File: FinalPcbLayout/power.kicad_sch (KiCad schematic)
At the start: 33 parts, among them Q1 NMOS, U4 AMS1117-3.3

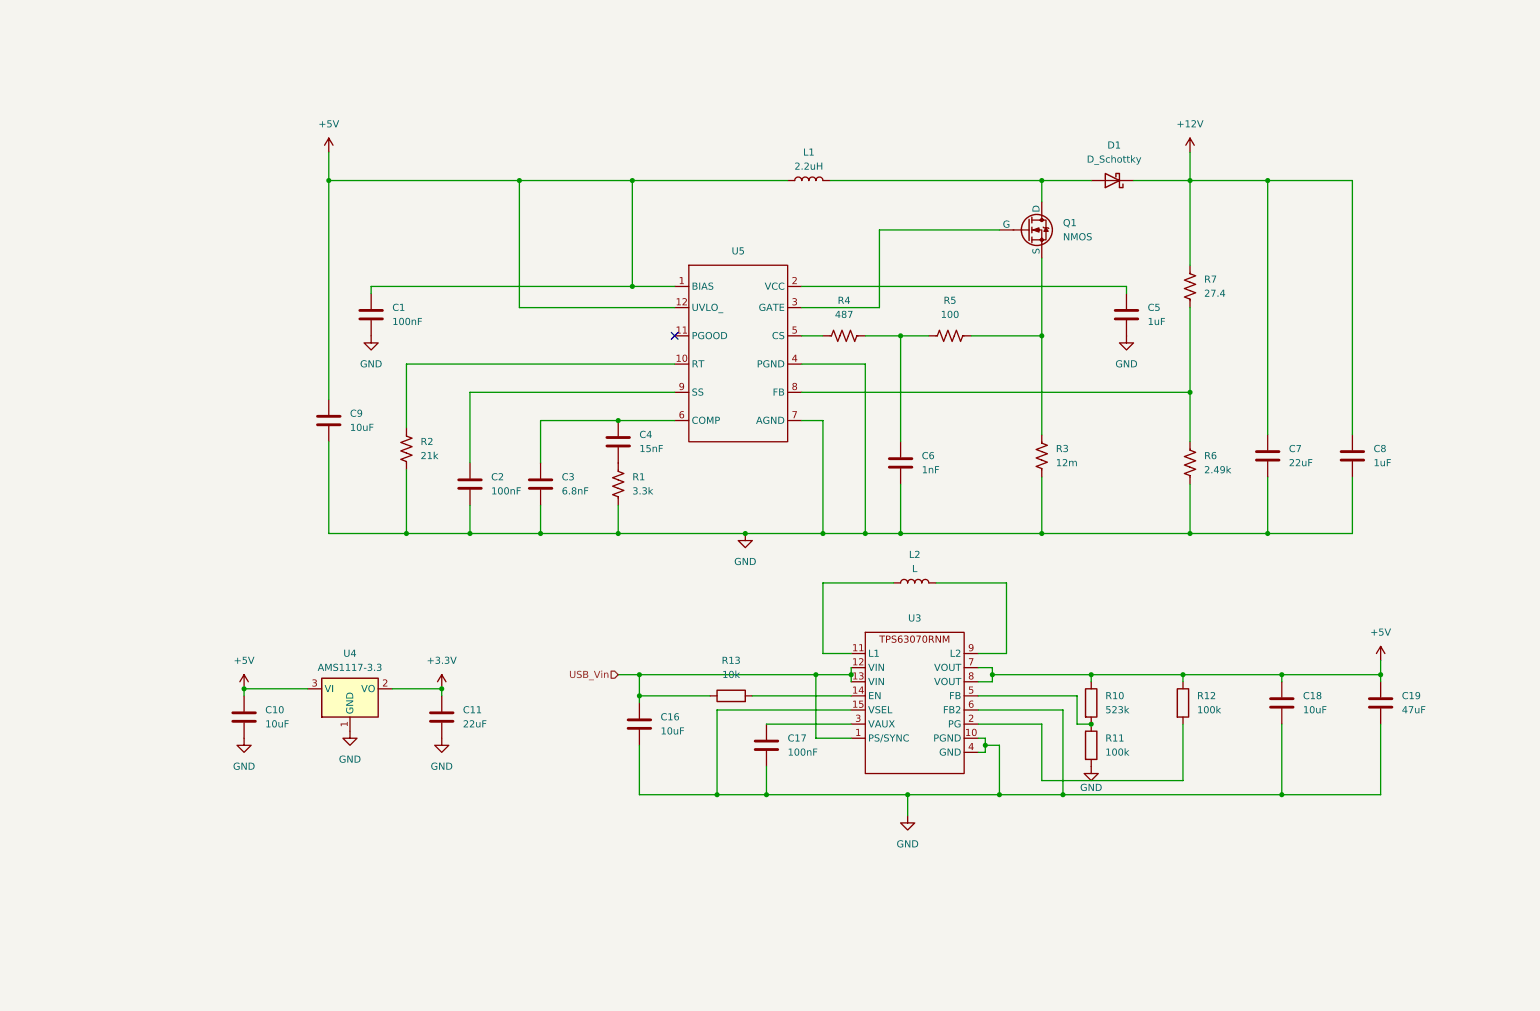
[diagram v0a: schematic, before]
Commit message: Part Finalization
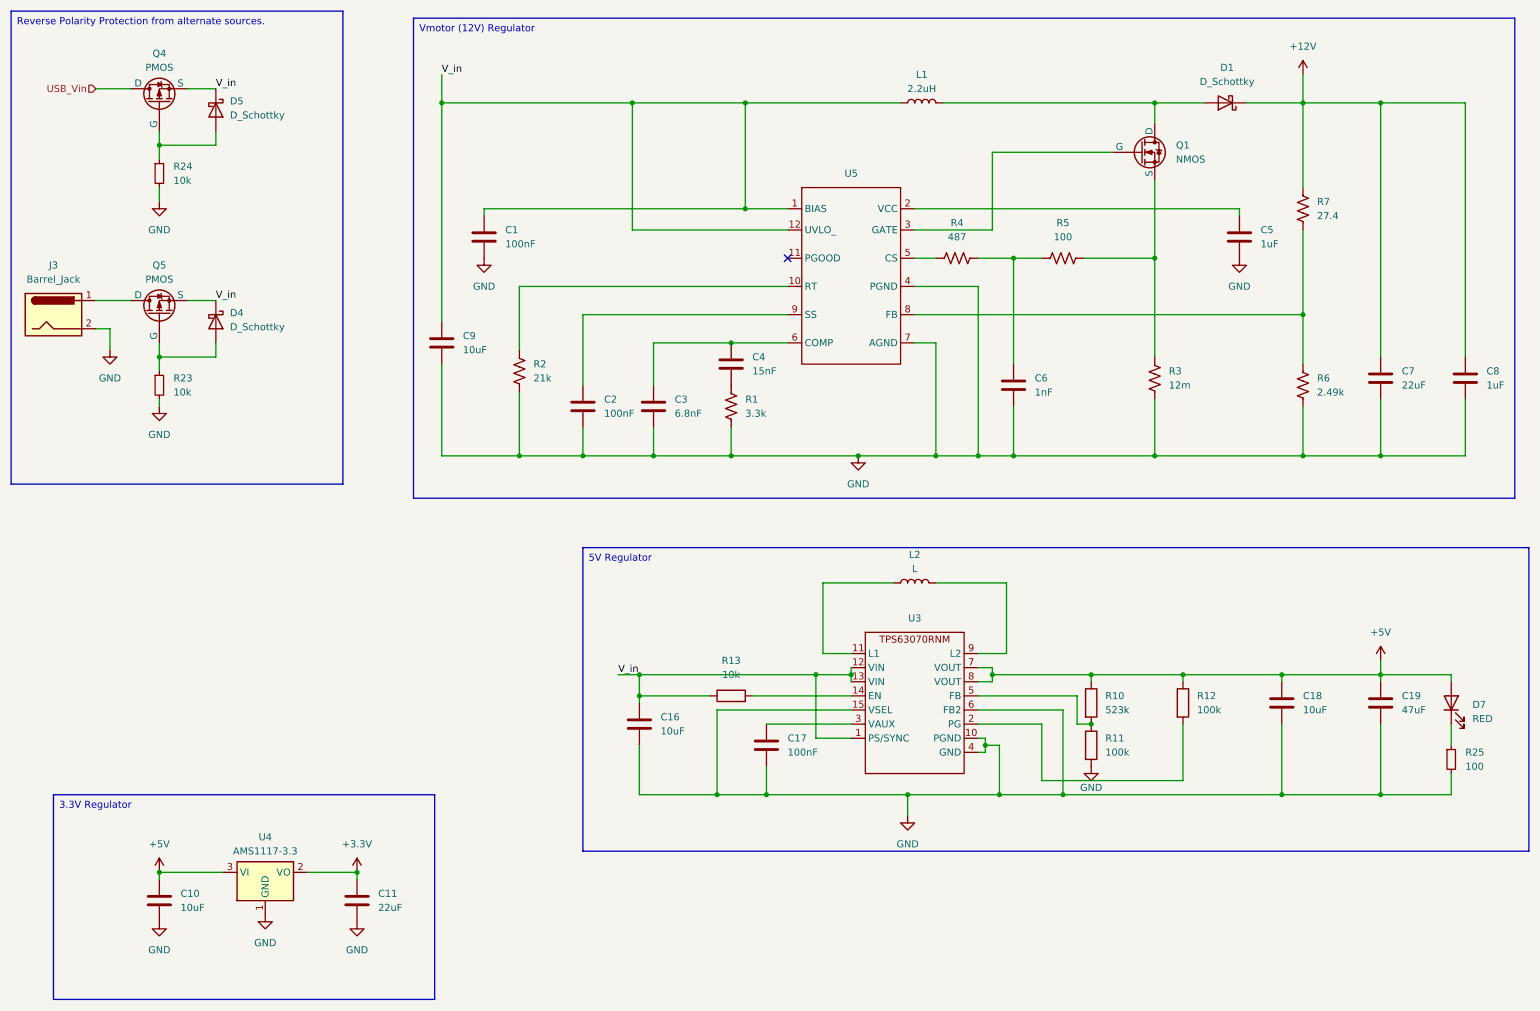
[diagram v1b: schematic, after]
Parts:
- added D4, D5: D_Schottky, symbol Device:D_Schottky
- added D7: RED, symbol Device:LED
- added J3: Barrel_Jack, Connector_BarrelJack:BarrelJack_GCT_DCJ200-10-A_Horizontal, symbol Connector:Barrel_Jack
- added Q4, Q5: PMOS, symbol Simulation_SPICE:PMOS
- added R23, R24: 10k, symbol Device:R_Small
- added R25: 100, symbol Device:R_Small
- D1: cost (none) -> .89; digikey_pn (none) -> SL42-E3/57TGITR-ND
- Q1: cost (none) -> .48; digikey_pn (none) -> 296-37193-6-ND
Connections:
- net +5V: now also D7.2 (A); no longer C1.2, C9.2, L1.1, U5.1 (BIAS), U5.12 (UVLO_)
- net GND: now also J3.2, R23.2, R24.2, R25.2
- net USB_Vin: now also Q4.1 (D); no longer C16.1, R13.1, U3.1 (PS/SYNC), U3.12 (VIN), U3.13 (VIN)
- new net: D7.1 (K), R25.1
- new net: D5.2 (A), Q4.2 (G), R24.1
- new net: D4.2 (A), Q5.2 (G), R23.1
- new net: J3.1, Q5.1 (D)
- new net V_in: C1.2, C16.1, C9.2, D4.1 (K), D5.1 (K), L1.1, Q4.3 (S), Q5.3 (S), R13.1, U3.1 (PS/SYNC), U3.12 (VIN), U3.13 (VIN), U5.1 (BIAS), U5.12 (UVLO_)
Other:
- moved on the sheet: C1, C10, C11, C2, C3, C4, C5, C6, C7, C8, C9, D1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
